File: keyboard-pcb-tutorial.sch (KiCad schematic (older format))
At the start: 24 parts, among them SW1 SW_Push, U1 ATmega32U4-AU, Y1 16MHz

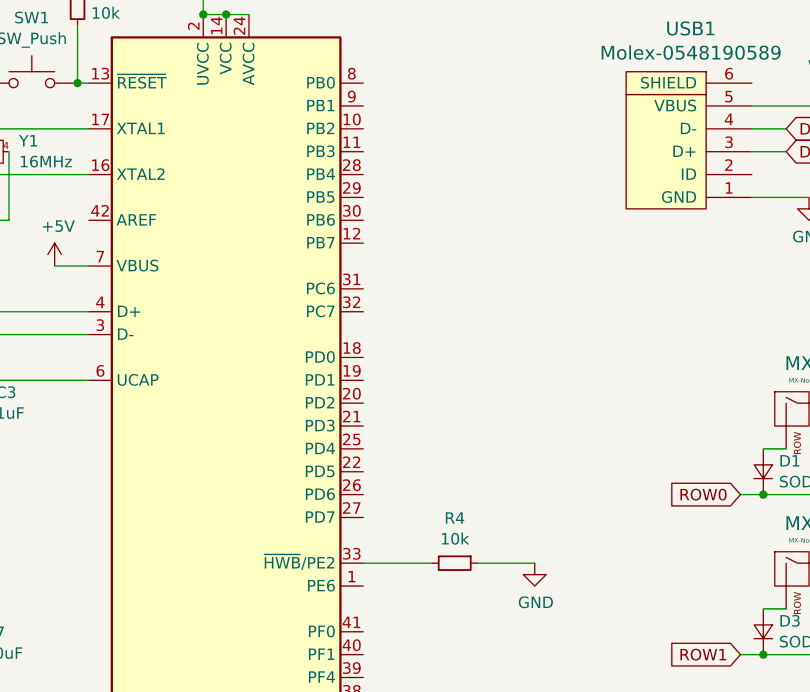
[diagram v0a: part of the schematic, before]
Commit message: Creating the PCB
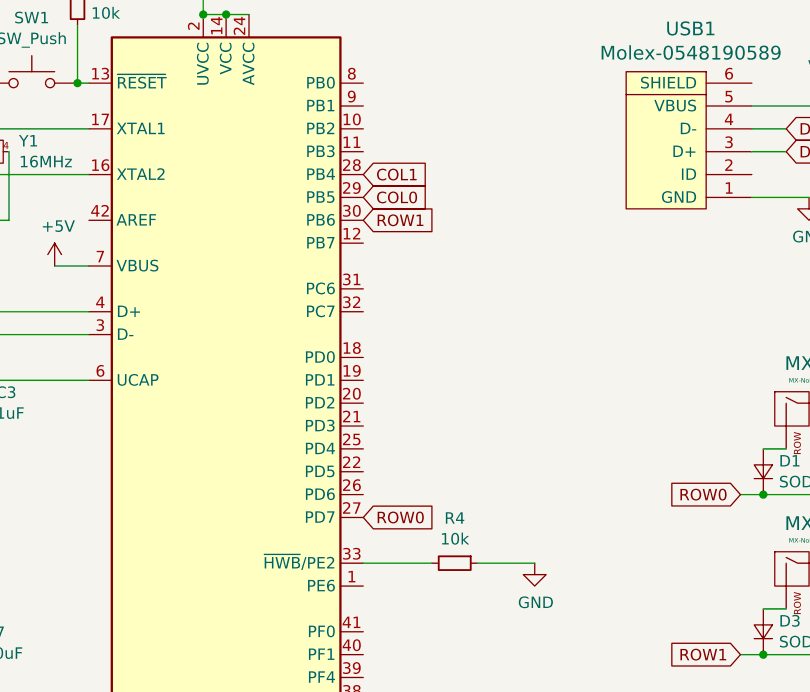
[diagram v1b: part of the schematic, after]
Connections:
- net COL0: now also U1.29 (PB5)
- net COL1: now also U1.28 (PB4)
- net ROW0: now also U1.27 (PD7)
- net ROW1: now also U1.30 (PB6)
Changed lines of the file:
@@
 Text GLabel 9150 2700 1    50   Input ~ 0
 COL1
+Text GLabel 6500 3400 2    50   Input ~ 0
+ROW0
+Text GLabel 6500 1900 2    50   Input ~ 0
+COL1
+Text GLabel 6500 2000 2    50   Input ~ 0
+COL0
+Text GLabel 6500 2100 2    50   Input ~ 0
+ROW1
 $EndSCHEMATC
